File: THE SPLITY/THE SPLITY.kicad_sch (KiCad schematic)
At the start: 66 parts, among them J1 Conn_01x02_Socket, U2 Nice_Nano_V2

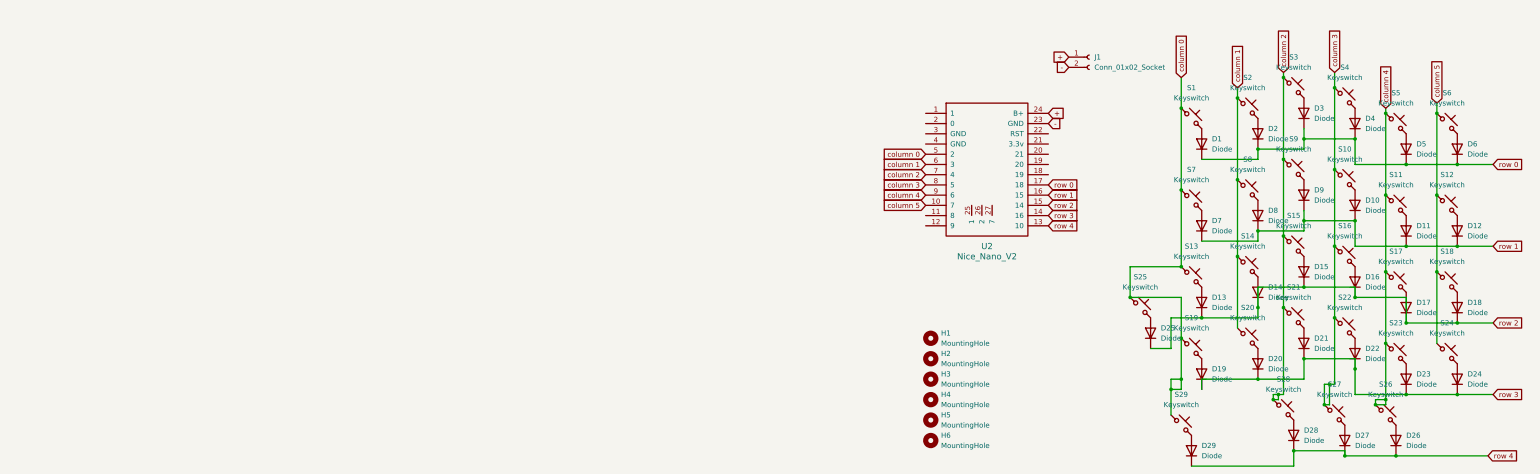
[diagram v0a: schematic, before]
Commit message: updated some stuff
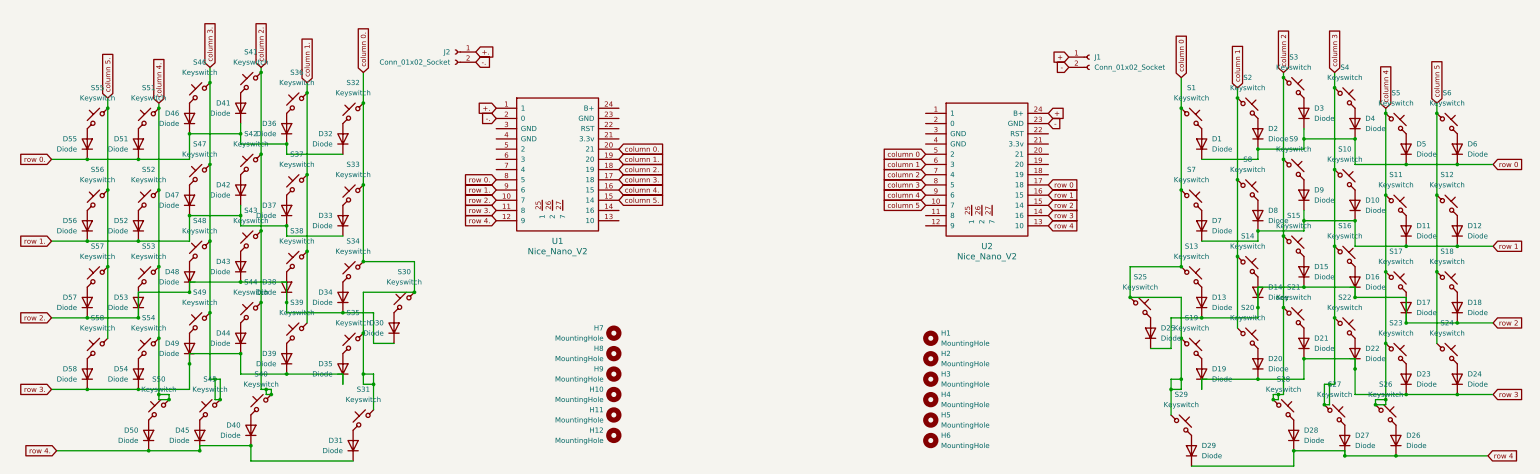
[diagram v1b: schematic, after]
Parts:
- added D30, D31, D32, D33, D34, D35, D36, D37, D38, D39, D40, D41, D42, D43, D44, D45, D46, D47, D48, D49, D50, D51, D52, D53, D54, D55, D56, D57, D58: Diode, ScottoKeebs_Components:Diode_DO-35, symbol ScottoKeebs:Placeholder_Diode
- added H10, H11, H12, H7, H8, H9: MountingHole, MountingHole:MountingHole_2.2mm_M2, symbol Mechanical:MountingHole
- added J2: Conn_01x02_Socket, Connector_JST:JST_XH_B2B-XH-AM_1x02_P2.50mm_Vertical, symbol Connector:Conn_01x02_Socket
- added S30, S31, S32, S33, S34, S35, S36, S37, S38, S39, S40, S41, S42, S43, S44, S45, S46, S47, S48, S49, S50, S51, S52, S53, S54, S55, S56, S57, S58: Keyswitch, ScottoKeebs_MX:MX_PCB_1.00u, symbol ScottoKeebs:Placeholder_Keyswitch
- added U1: Nice_Nano_V2, ScottoKeebs_MCU:Nice_Nano_V2_Flipped, symbol ScottoKeebs:MCU_Nice_Nano_V2
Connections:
- new net: D35.2 (A), S35.2
- new net: D58.2 (A), S58.2
- new net: D57.2 (A), S57.2
- new net: D46.2 (A), S46.2
- new net: D37.2 (A), S37.2
- new net: D40.2 (A), S40.2
- new net: D45.2 (A), S45.2
- new net: D49.2 (A), S49.2
- new net: D33.2 (A), S33.2
- new net: D42.2 (A), S42.2
- new net: D34.2 (A), S34.2
- new net: D55.2 (A), S55.2
- new net: D43.2 (A), S43.2
- new net: D32.2 (A), S32.2
- new net: D47.2 (A), S47.2
- new net: D44.2 (A), S44.2
- new net: D30.2 (A), S30.2
- new net: D53.2 (A), S53.2
- new net: D36.2 (A), S36.2
- new net: D39.2 (A), S39.2
- new net: D50.2 (A), S50.2
- new net: D51.2 (A), S51.2
- new net: D48.2 (A), S48.2
- new net: D56.2 (A), S56.2
- new net: D38.2 (A), S38.2
- new net: D41.2 (A), S41.2
- new net: D54.2 (A), S54.2
- new net: D52.2 (A), S52.2
- new net: D31.2 (A), S31.2
- new net +.: J2.1 (Pin_1), U1.1
- new net -.: J2.2 (Pin_2), U1.2 (0)
- new net column 0.: S30.1, S31.1, S32.1, S33.1, S34.1, S35.1, U1.20 (21)
- new net column 1.: S36.1, S37.1, S38.1, S39.1, U1.19 (20)
- new net column 2.: S40.1, S41.1, S42.1, S43.1, S44.1, U1.18 (19)
- new net column 3.: S45.1, S46.1, S47.1, S48.1, S49.1, U1.17 (18)
- new net column 4.: S50.1, S51.1, S52.1, S53.1, S54.1, U1.16 (15)
- new net column 5.: S55.1, S56.1, S57.1, S58.1, U1.15 (14)
- new net row 0.: D32.1 (K), D36.1 (K), D41.1 (K), D46.1 (K), D51.1 (K), D55.1 (K), U1.8 (5)
- new net row 1.: D33.1 (K), D37.1 (K), D42.1 (K), D47.1 (K), D52.1 (K), D56.1 (K), U1.9 (6)
- new net row 2.: D30.1 (K), D34.1 (K), D38.1 (K), D43.1 (K), D48.1 (K), D53.1 (K), D57.1 (K), U1.10 (7)
- new net row 3.: D35.1 (K), D39.1 (K), D44.1 (K), D49.1 (K), D54.1 (K), D58.1 (K), U1.11 (8)
- new net row 4.: D31.1 (K), D40.1 (K), D45.1 (K), D50.1 (K), U1.12 (9)
